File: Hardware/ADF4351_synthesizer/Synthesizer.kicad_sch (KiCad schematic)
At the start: 53 parts, among them J3 SMA-J-P-H-ST-EM1, J4 SMA-J-P-H-ST-EM1, J5 SMA-J-P-H-ST-EM1, U3 ADM7150ARDZ-3.3-R7, U4 ADF4351, X1 XO32

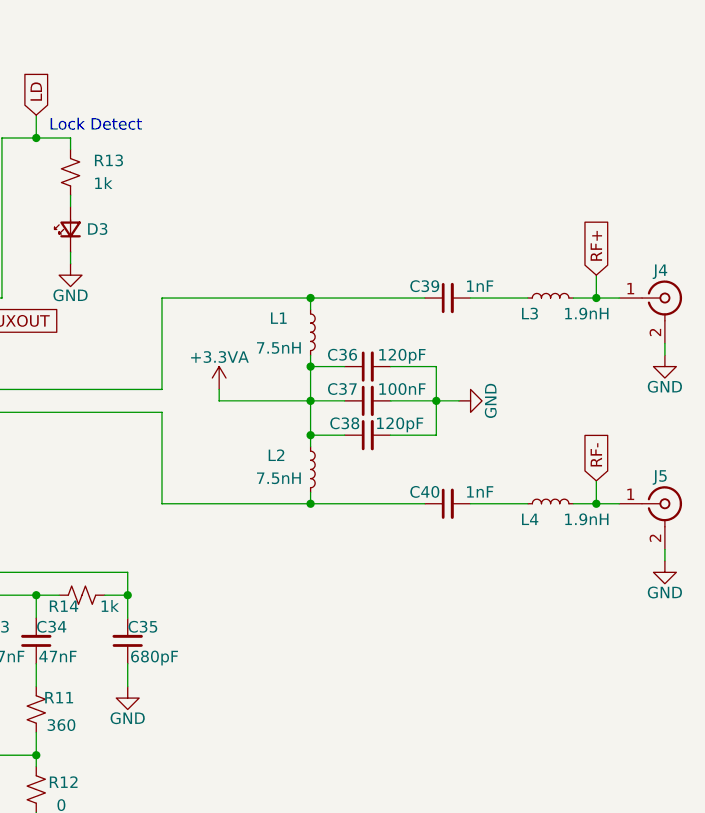
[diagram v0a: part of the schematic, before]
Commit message: Updating board
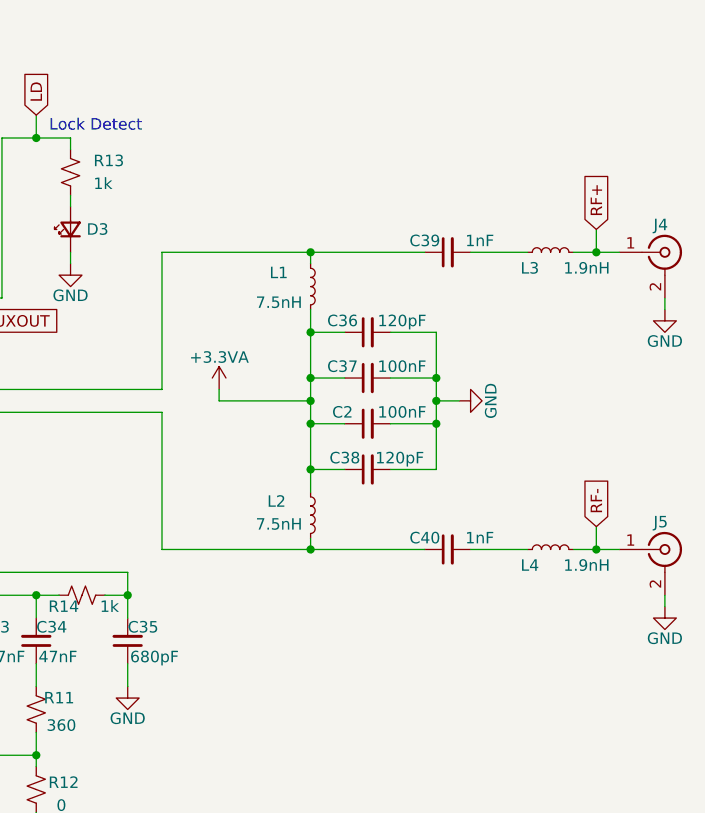
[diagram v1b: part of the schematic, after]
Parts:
- added C2: 100nF, Capacitor_SMD:C_0402_1005Metric, symbol Device:C_Small
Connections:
- net +3.3VA: now also C2.1
- net GND: now also C2.2
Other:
- moved on the sheet: C36, C37, C38, C39, C40, J4, J5, L1, L2, L3, L4
